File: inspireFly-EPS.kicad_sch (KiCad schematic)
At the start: 98 parts, among them J1 USB4085-GF-A_REVB, J2 Conn_01x02_Pin, Q10 SQJA62EP-T1_GE3, Q3 SQJA62EP-T1_GE3, Q4 SQJA62EP-T1_GE3, Q5 SQJA62EP-T1_GE3, Q6 SQJA62EP-T1_GE3, Q7 SQJA62EP-T1_GE3, Q8 SQJA62EP-T1_GE3, Q9 SQJA62EP-T1_GE3, U1 STM32U575RIT6, U2 BQ25750RRVR, U3 TCAN332DCNR, U4 MAX77504AAFC+T, U5 INA180A3IDBVT, U6 INA180A3IDBVT, U7 INA180A3IDBVT, U8 TPS63070RNMR, U9 TPS63070RNMR

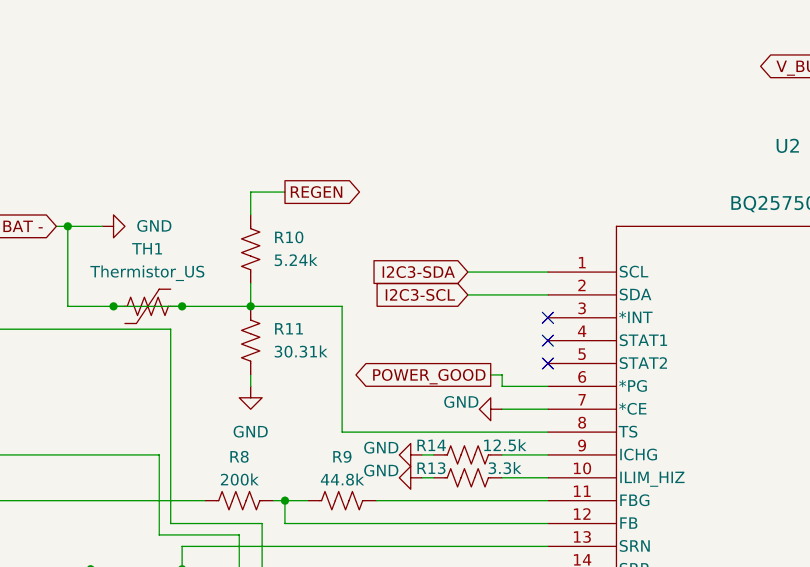
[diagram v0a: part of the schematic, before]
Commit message: Routing fixes
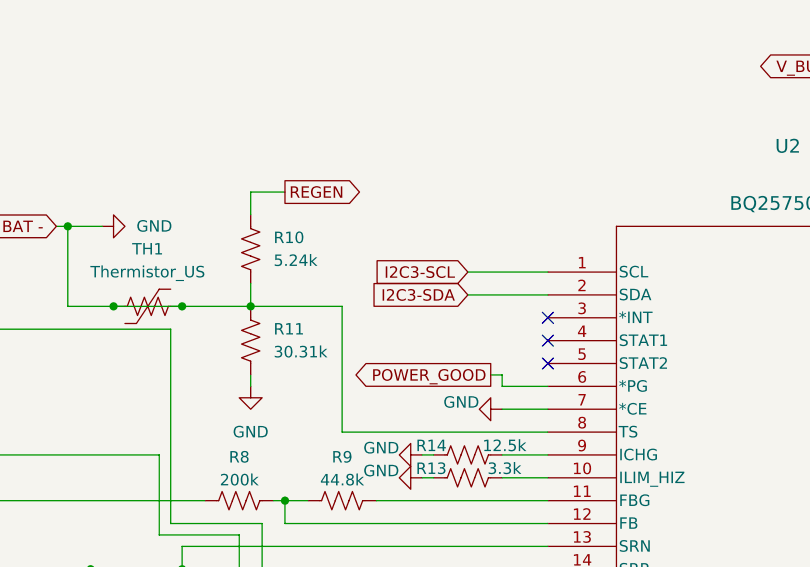
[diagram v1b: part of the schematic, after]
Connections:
- net I2C3-SCL: now also U2.1 (SCL); no longer U2.2 (SDA)
- net I2C3-SDA: now also U2.2 (SDA); no longer U2.1 (SCL)
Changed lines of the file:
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@@
 	(wire
 		(pts
+			(xy 109.22 341.63) (xy 118.11 341.63)
+		)
+		(stroke
+			(width 0)
+			(type default)
+		)
+	)
+	(wire
+		(pts
 			(xy 44.45 245.11) (xy 46.99 245.11)
 		)
@@
 	(wire
 		(pts
-			(xy 109.22 341.63) (xy 118.11 341.63)
-		)
-		(stroke
-			(width 0)
-			(type default)
-		)
-	)
-	(wire
-		(pts
 			(xy 459.74 290.83) (xy 459.74 294.64)
 		)
@@
 	(wire
 		(pts
-			(xy 386.08 234.95) (xy 396.24 234.95)
+			(xy 109.22 339.09) (xy 118.11 339.09)
 		)
 		(stroke
@@
 	(wire
 		(pts
-			(xy 170.18 35.56) (xy 170.18 39.37)
+			(xy 386.08 234.95) (xy 396.24 234.95)
 		)
 		(stroke
@@
 	(wire
 		(pts
-			(xy 85.09 342.9) (xy 77.47 342.9)
+			(xy 170.18 35.56) (xy 170.18 39.37)
 		)
 		(stroke
@@
 	(wire
 		(pts
-			(xy 69.85 342.9) (xy 64.77 342.9)
+			(xy 85.09 342.9) (xy 77.47 342.9)
 		)
 		(stroke
@@
 	(wire
 		(pts
-			(xy 321.31 220.98) (xy 327.66 220.98)
+			(xy 69.85 342.9) (xy 64.77 342.9)
 		)
 		(stroke
@@
 	(wire
 		(pts
-			(xy 173.99 382.27) (xy 203.2 382.27)
+			(xy 321.31 220.98) (xy 327.66 220.98)
 		)
 		(stroke
@@
 	(wire
 		(pts
-			(xy 271.78 224.79) (xy 271.78 222.25)
+			(xy 173.99 382.27) (xy 203.2 382.27)
 		)
 		(stroke
@@
 	(wire
 		(pts
-			(xy 256.54 347.98) (xy 264.16 347.98)
+			(xy 271.78 224.79) (xy 271.78 222.25)
 		)
 		(stroke
@@
 	(wire
 		(pts
-			(xy 109.22 339.09) (xy 118.11 339.09)
+			(xy 256.54 347.98) (xy 264.16 347.98)
 		)
 		(stroke
@@
 	(global_label "I2C3-SCL"
 		(shape input)
-		(at 109.22 341.63 180)
+		(at 109.22 339.09 180)
 		(fields_autoplaced yes)
 		(effects
@@
 		)
 		(property "Intersheetrefs" "${INTERSHEET_REFS}"
-			(at 96.861 341.63 0)
+			(at 96.861 339.09 0)
 			(effects
 				(font
@@
 	(global_label "I2C3-SDA"
 		(shape input)
-		(at 109.22 339.09 180)
+		(at 109.22 341.63 180)
 		(fields_autoplaced yes)
 		(effects
@@
 		)
 		(property "Intersheetrefs" "${INTERSHEET_REFS}"
-			(at 96.8005 339.09 0)
+			(at 96.8005 341.63 0)
 			(effects
 				(font
